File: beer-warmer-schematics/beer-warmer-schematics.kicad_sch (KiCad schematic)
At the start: 40 parts, among them J1 USB_C_Receptacle_6P, J2 Screw_Terminal_01x02, J3 Conn_01x07_Socket, J4 Conn_01x07_Socket, J5 Conn_01x04_Pin, J6 Screw_Terminal_01x03, Q1 AOD4184A, U2 TPS5430DDA, U3 CH224K, U4 INA219AxDCN

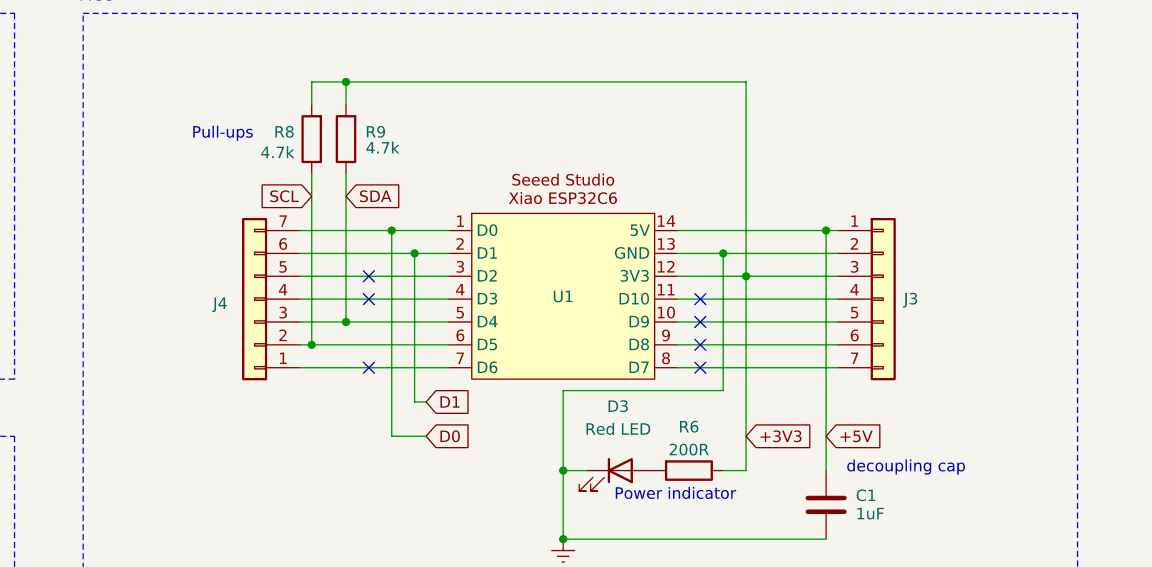
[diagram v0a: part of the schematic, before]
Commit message: routing overhaul
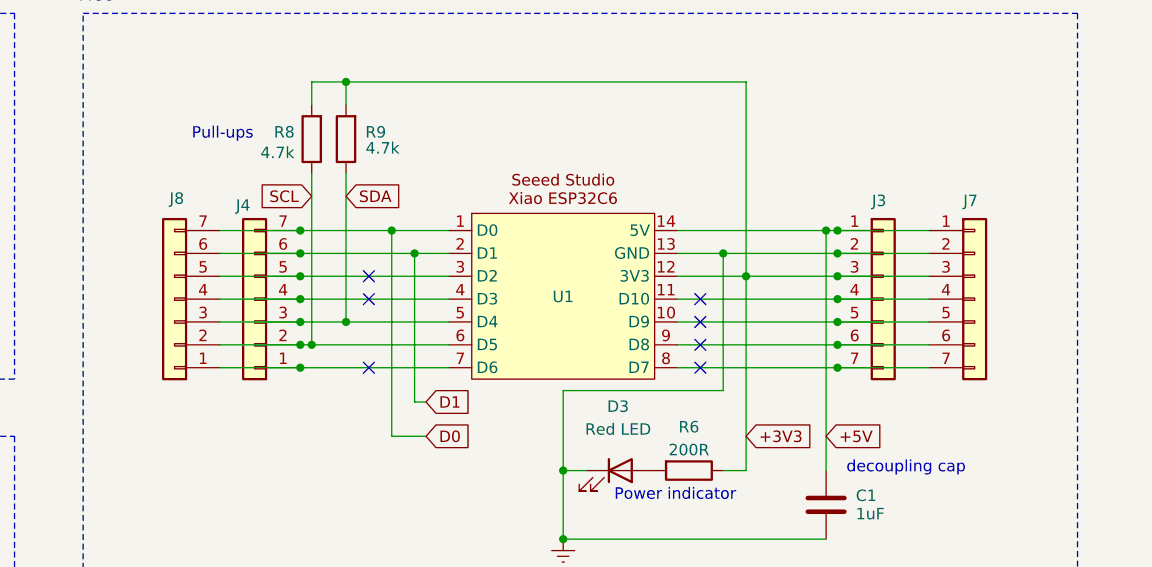
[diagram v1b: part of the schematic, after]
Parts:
- added J7, J8: Conn_01x07_Socket, Connector_PinHeader_2.54mm:PinHeader_1x07_P2.54mm_Vertical, symbol Connector_Generic:Conn_01x07
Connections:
- net +3V3: now also J7.3 (Pin_3)
- net +5V: now also J7.1 (Pin_1)
- net D0: now also J8.7 (Pin_7)
- net D1: now also J8.6 (Pin_6)
- net GND: now also J7.2 (Pin_2)
- net SCL: now also J8.2 (Pin_2)
- net SDA: now also J8.3 (Pin_3)
- net at J3.5 (Pin_5), U1.10 (D9): now also J7.5 (Pin_5)
- net at J3.4 (Pin_4), U1.11 (D10): now also J7.4 (Pin_4)
- net at J4.5 (Pin_5), U1.3 (D2): now also J8.5 (Pin_5)
- net at J4.4 (Pin_4), U1.4 (D3): now also J8.4 (Pin_4)
- net at J4.1 (Pin_1), U1.7 (D6): now also J8.1 (Pin_1)
- net at J3.7 (Pin_7), U1.8 (D7): now also J7.7 (Pin_7)
- net at J3.6 (Pin_6), U1.9 (D8): now also J7.6 (Pin_6)
